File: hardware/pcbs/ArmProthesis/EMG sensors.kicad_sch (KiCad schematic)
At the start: 30 parts, among them IC1 INA128, J2 Conn_01x01_Pin, J3 Conn_01x03_Pin, J4 Conn_01x01_Pin, U6 OPA2188AIDR, U7 OPA188AIDR

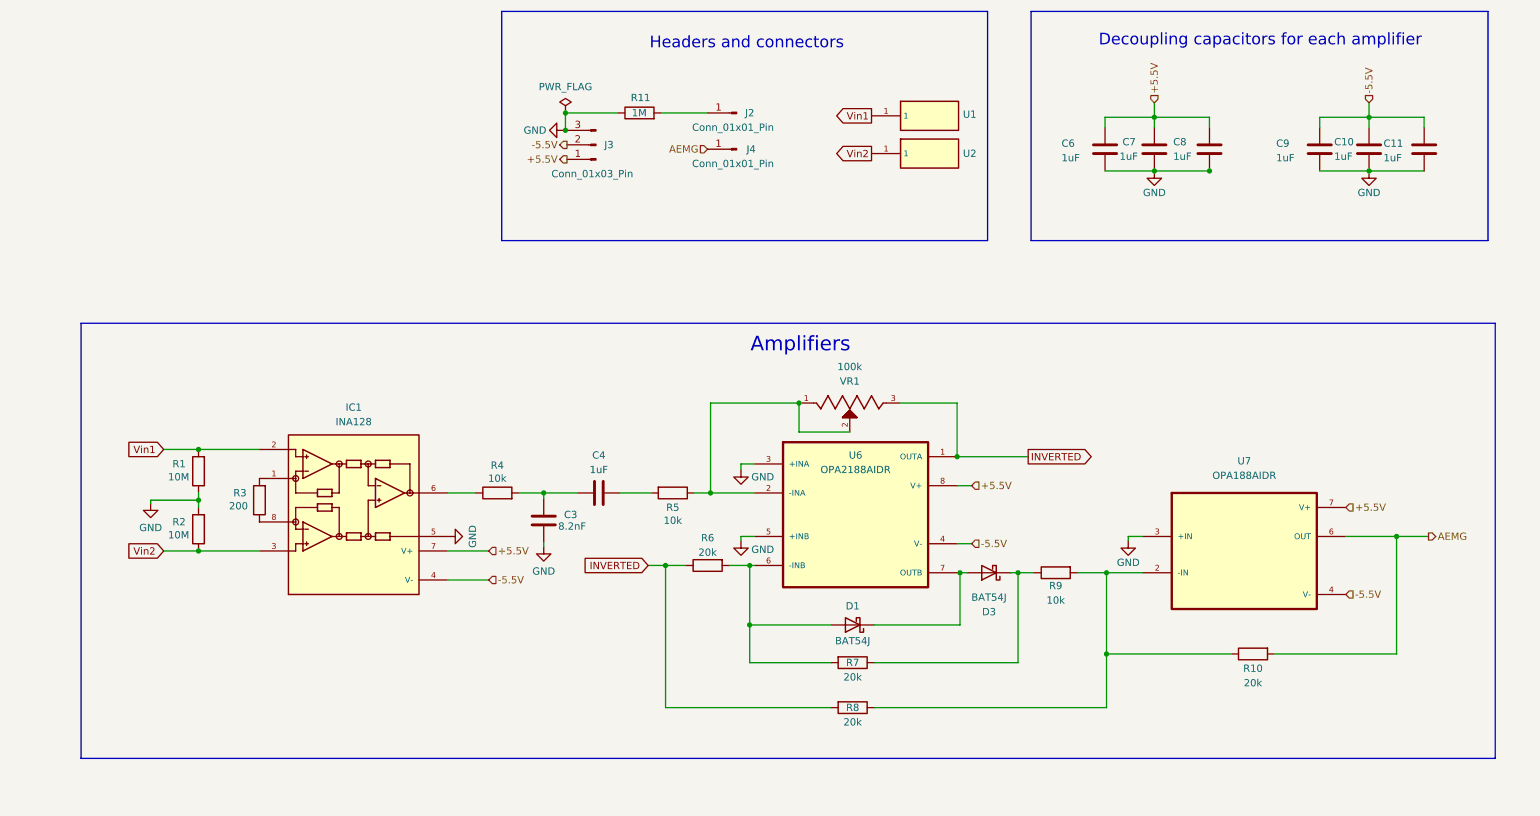
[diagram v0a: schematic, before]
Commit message: .
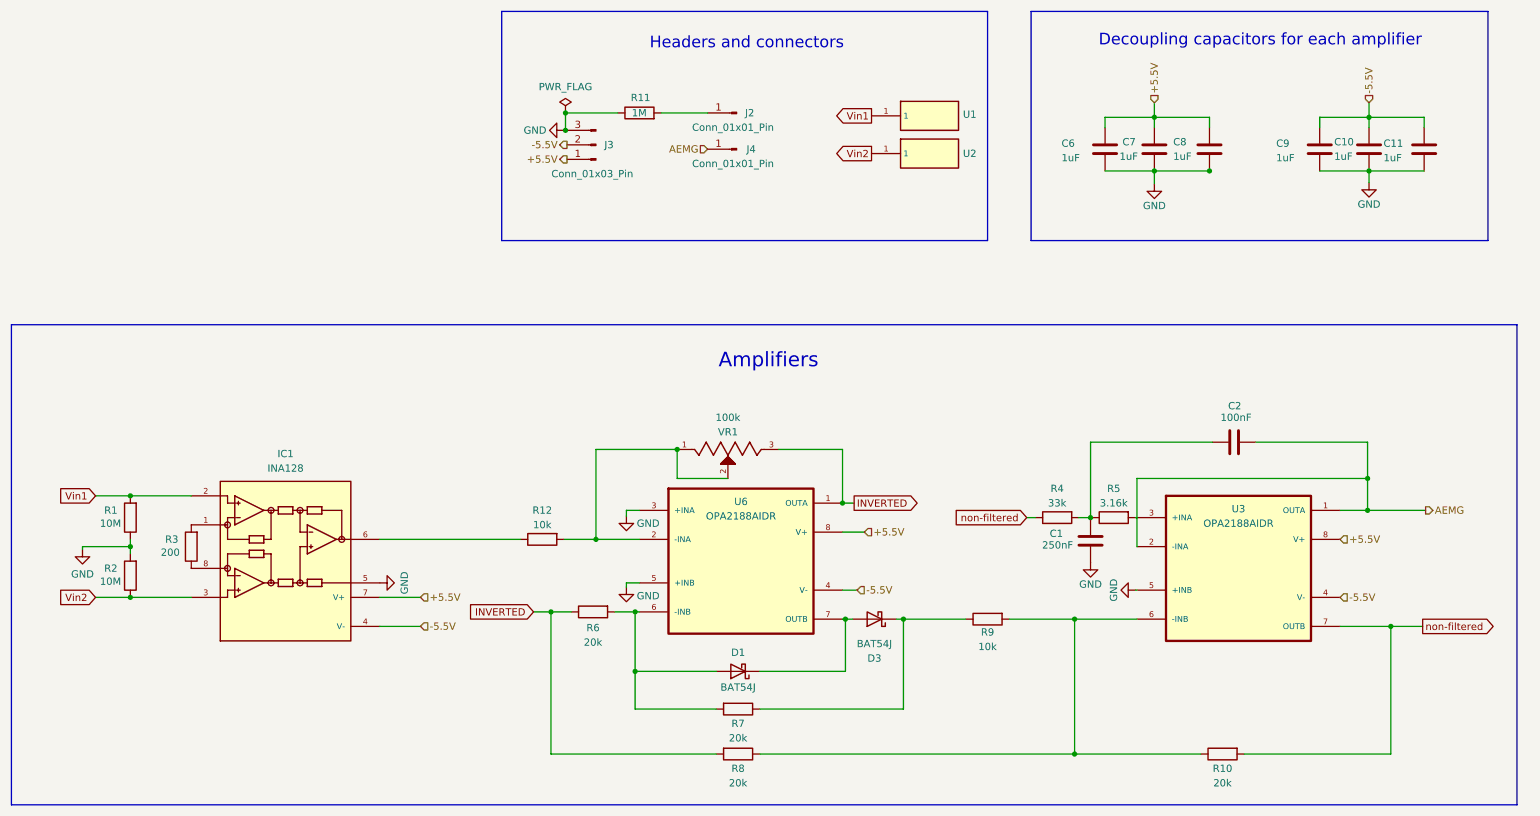
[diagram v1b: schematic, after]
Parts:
- removed C3: 8.2nF, Capacitor_SMD:C_0603_1608Metric_Pad1.08x0.95mm_HandSolder, symbol Device:C
- removed C4: 1uF, Capacitor_SMD:C_0603_1608Metric_Pad1.08x0.95mm_HandSolder, symbol Device:C
- removed U7: OPA188AIDR, OP AMPS:OPA188, symbol OP AMPS:OPA188AIDR
- added C1: 250nF, Resistor_SMD:R_0402_1005Metric, symbol Device:C
- added C2: 100nF, Resistor_SMD:R_0402_1005Metric, symbol Device:C
- added R12: 10k, Resistor_SMD:R_0402_1005Metric, symbol Device:R
- added U3: OPA2188AIDR, OP AMPS:OPA2188, symbol OP AMPS:OPA2188AIDR
- R10, R3, R6, R7, R8, R9: footprint Resistor_SMD:R_0603_1608Metric_Pad0.98x0.95mm_HandSolder -> Resistor_SMD:R_0402_1005Metric
- R4: value 10k -> 33k; footprint Resistor_SMD:R_0603_1608Metric_Pad0.98x0.95mm_HandSolder -> Resistor_SMD:R_0402_1005Metric
- R5: value 10k -> 3.16k; footprint Resistor_SMD:R_0603_1608Metric_Pad0.98x0.95mm_HandSolder -> Resistor_SMD:R_0402_1005Metric
- U6: footprint OP AMPS:ОПА2188AIDR -> OP AMPS:OPA2188
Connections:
- net +5.5V: now also U3.8 (V+)
- net -5.5V: now also U3.4 (V-)
- net AEMG: now also C2.1, U3.1 (OUTA), U3.2 (-INA); no longer R10.2
- net GND: now also C1.1, U3.5 (+INB)
- net at IC1.6: now also R12.1; no longer R4.1
- net at R4.2: now also R5.1, C1.2, C2.2
- net at R10.1, R8.1, R9.2: now also U3.6 (-INB)
- net at U6.2 (-INA), VR1.1, VR1.2: now also R12.2; no longer R5.1
- net at R5.2: now also U3.3 (+INA)
- new net non-filtered: R10.2, R4.1, U3.7 (OUTB)
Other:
- moved on the sheet: D1, D3, IC1, R1, R10, R2, R3, R6, R7, R8, R9, U6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

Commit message: updates
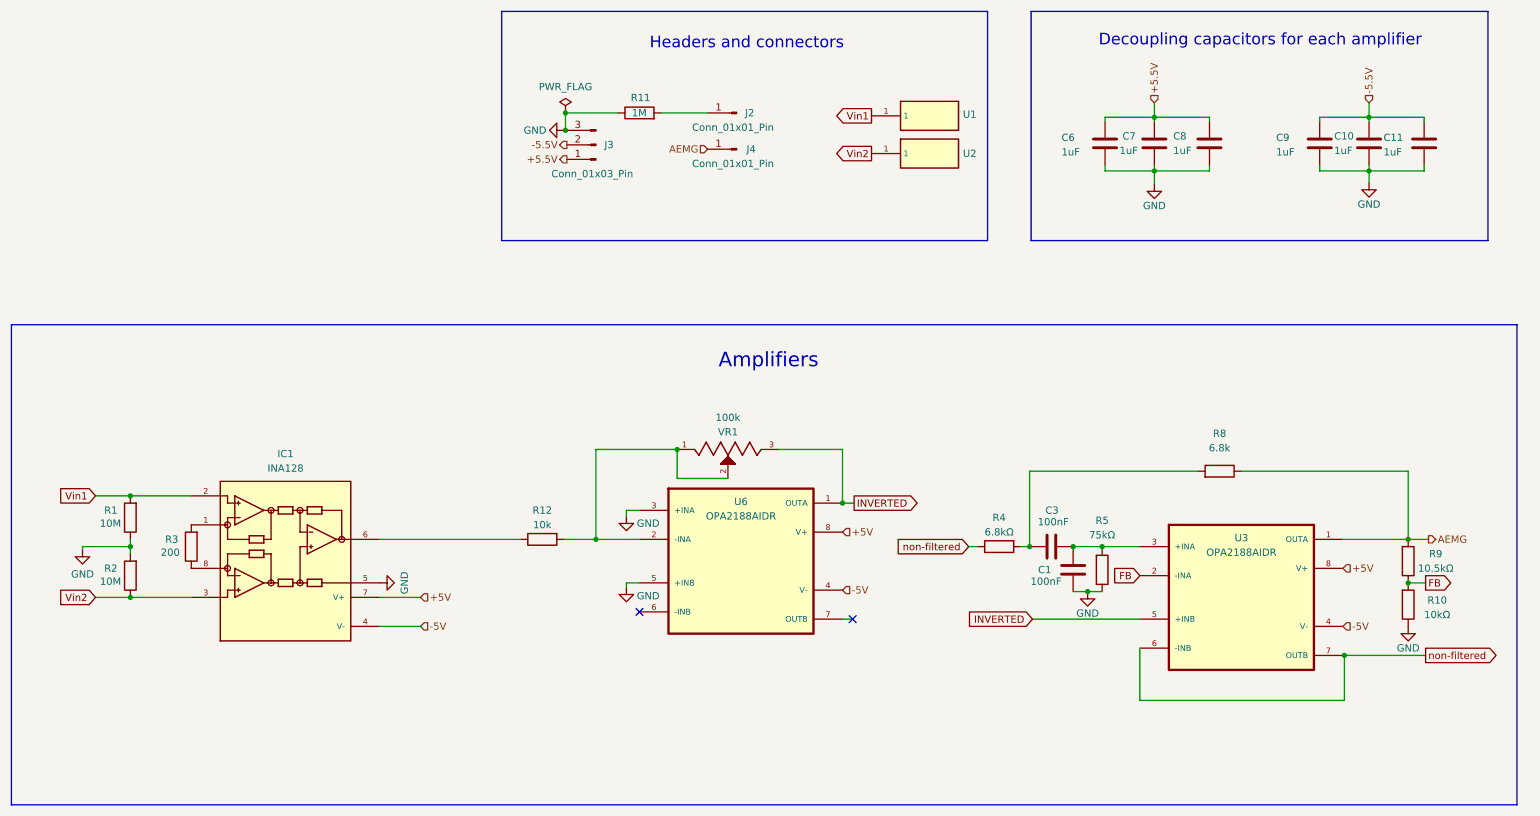
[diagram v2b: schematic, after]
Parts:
- removed C2: 100nF, Resistor_SMD:R_0402_1005Metric, symbol Device:C
- removed D1, D3: BAT54J, Diode_SMD:D_SOD-323F, symbol Diode:BAT54J
- removed R6, R7: 20k, Resistor_SMD:R_0402_1005Metric, symbol Device:R
- added C3: 100nF, Resistor_SMD:R_0402_1005Metric, symbol Device:C
- C1: value 250nF -> 100nF; LCSC (none) -> C307331
- C10, C11, C6, C7, C8, C9: footprint Capacitor_SMD:C_0603_1608Metric_Pad1.08x0.95mm_HandSolder -> Resistor_SMD:R_0603_1608Metric; LCSC (none) -> C15849
- IC1: LCSC (none) -> C22233
- J3: LCSC (none) -> C514175
- R1, R2: footprint Resistor_SMD:R_0603_1608Metric_Pad0.98x0.95mm_HandSolder -> Resistor_SMD:R_0603_1608Metric; LCSC (none) -> C7250
- R10: value 20k -> 10kΩ; LCSC (none) -> C25850
- R11: footprint Resistor_SMD:R_0603_1608Metric_Pad0.98x0.95mm_HandSolder -> Resistor_SMD:R_0603_1608Metric; LCSC (none) -> C22935
- R12: LCSC (none) -> C25744
- R3: LCSC (none) -> C25087
- R4: value 33k -> 6.8kΩ; LCSC (none) -> C25917
- R5: value 3.16k -> 75kΩ; LCSC (none) -> C25798
- R8: value 20k -> 6.8k; LCSC (none) -> C25917
- R9: value 10k -> 10.5kΩ; LCSC (none) -> C173943
- U3, U6: LCSC (none) -> C17271
- VR1: LCSC (none) -> C48084
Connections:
- net +5.5V: no longer IC1.7 (V+), U3.8 (V+), U6.8 (V+)
- net -5.5V: no longer IC1.4 (V-), U3.4 (V-), U6.4 (V-)
- net AEMG: now also R8.1, R9.2; no longer U3.2 (-INA)
- net GND: now also R10.1, R5.1; no longer U3.5 (+INB)
- net INVERTED: now also U3.5 (+INB); no longer R8.2
- net non-filtered: now also U3.6 (-INB); no longer R10.2
- net at R5.2, U3.3 (+INA): now also C1.2, C3.1
- net FB: now reaches R9.1
- net FB: now also R10.2, U3.2 (-INA)
- new net: C3.2, R4.2, R8.2
- new net +5V: IC1.7 (V+), U3.8 (V+), U6.8 (V+)
- new net -5V: IC1.4 (V-), U3.4 (V-), U6.4 (V-)
- no-connect marks 0 -> 2
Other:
- moved on the sheet: C1, C10, C11, C6, C7, C8, C9, R4, R5, U3
